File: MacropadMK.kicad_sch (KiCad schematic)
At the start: 43 parts, among them J1 BME280, SHT40 Module, J10 SCD40 Module, J11 Conn_01x03, J12 Conn_01x03, J13 SCD40 Module, J14 BME280, SHT40 Module, J15 mmWave Connector, J16 mmWave Connector, J17 mmWave Connector, J2 SCD40 Module, J3 Conn_01x02, J4 Qwiic_Vertical, J5 Conn_01x02, J6 Conn_01x02, J7 Conn_01x03, J8 Conn_01x03, J9 VL53L0X Module, Q1 PT19-21C, SW1 SW_Push, U5 TLP175A

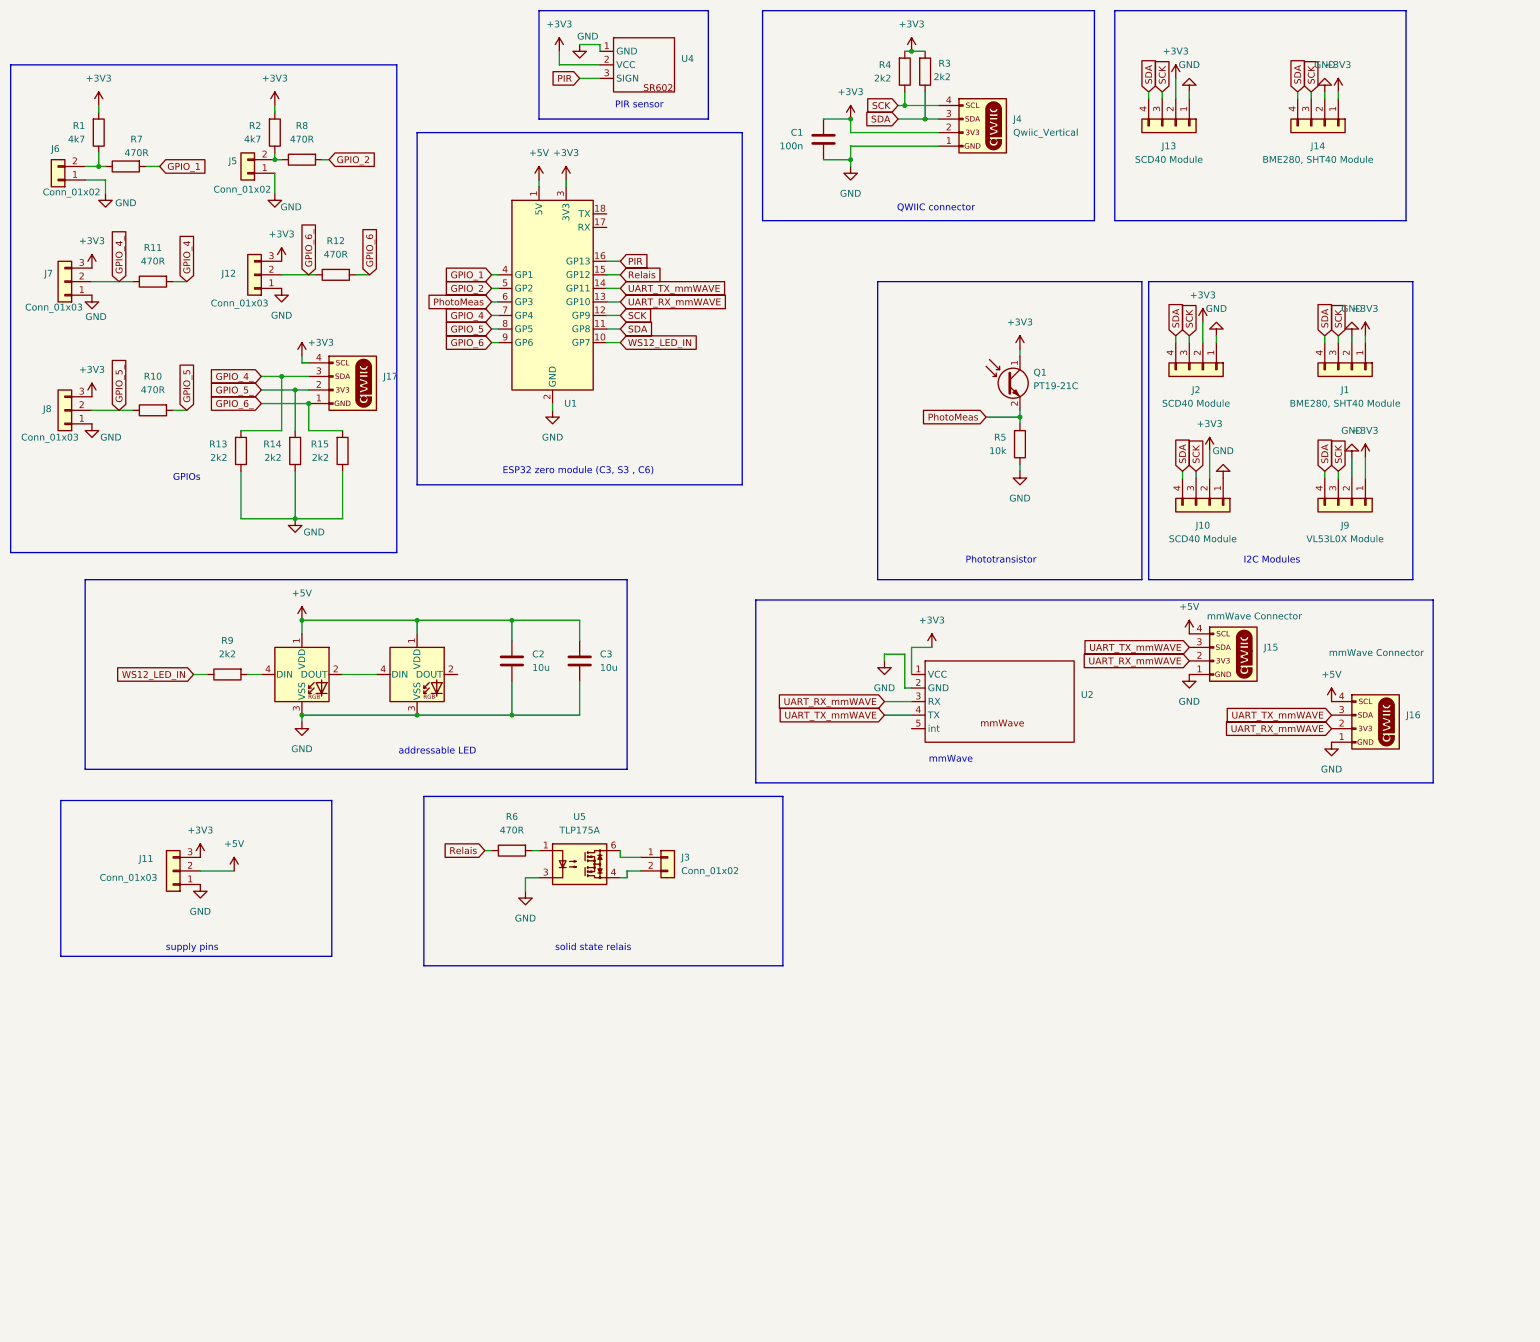
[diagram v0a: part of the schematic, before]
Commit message: added librarys
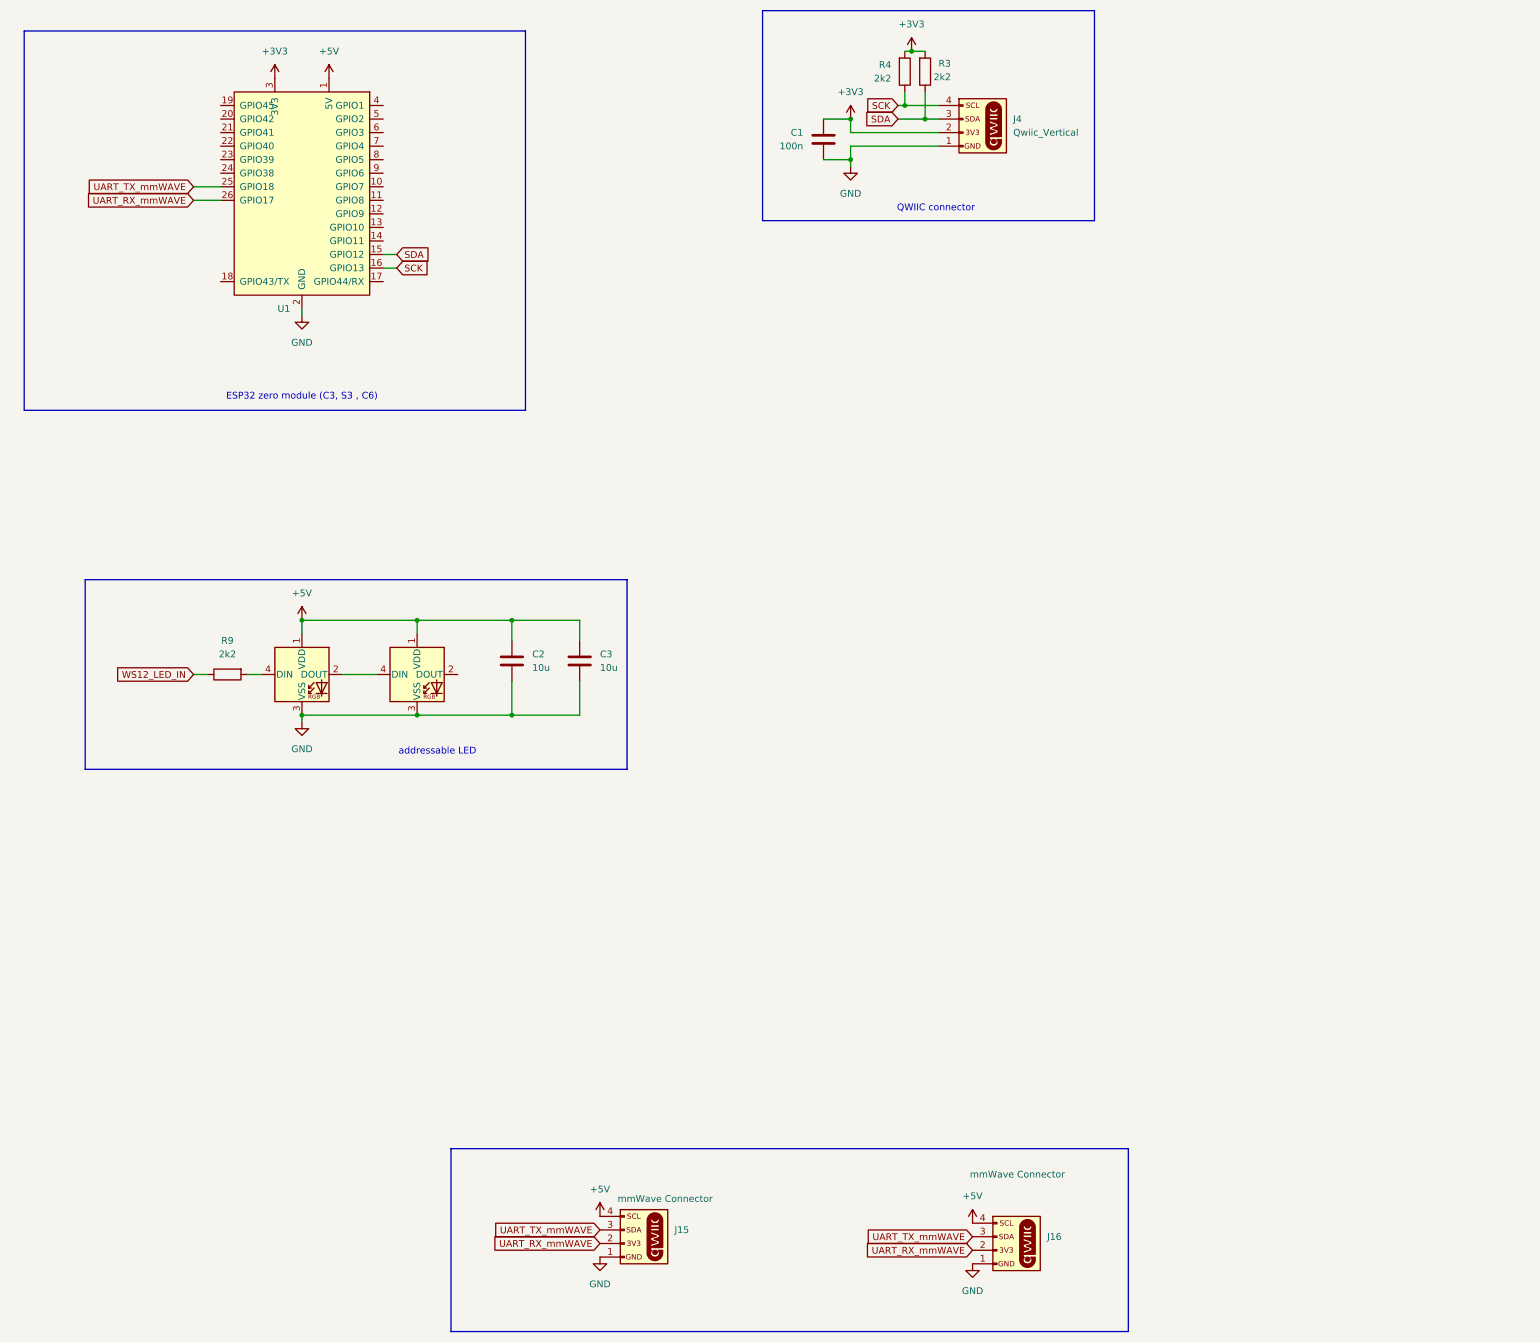
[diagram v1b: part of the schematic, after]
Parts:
- removed J1, J14: BME280, SHT40 Module, PCM_SparkFun-Connector:1x04_P2.54mm, symbol PCM_SparkFun-Connector:Conn_01x04_P2.54mm
- removed J10, J13, J2: SCD40 Module, PCM_SparkFun-Connector:1x04_P2.54mm, symbol PCM_SparkFun-Connector:Conn_01x04_P2.54mm
- removed J11, J12, J7, J8: Conn_01x03, PCM_SparkFun-Connector:1x03_P2.54mm, symbol PCM_SparkFun-Connector:Conn_01x03_P2.54mm
- removed J17: mmWave Connector, PCM_SparkFun-Connector:JST_1x04_P1.0mm_Vertical_SMD, symbol PCM_SparkFun-Connector:Qwiic_Vertical
- removed J3, J5, J6: Conn_01x02, PCM_SparkFun-Connector:1x02_P2.54mm, symbol PCM_SparkFun-Connector:Conn_01x02_P2.54mm
- removed J9: VL53L0X Module, PCM_SparkFun-Connector:1x04_P2.54mm, symbol PCM_SparkFun-Connector:Conn_01x04_P2.54mm
- removed Q1: PT19-21C, LED_SMD:LED_0603_1608Metric, symbol Device:Q_Photo_NPN
- removed R1, R2: 4k7, Resistor_SMD:R_0805_2012Metric, symbol Device:R
- removed R10, R11, R12, R6, R7, R8: 470R, Resistor_SMD:R_0805_2012Metric, symbol Device:R
- removed R13, R14, R15: 2k2, Resistor_SMD:R_0805_2012Metric, symbol Device:R
- removed R5: 10k, Resistor_SMD:R_0805_2012Metric, symbol Device:R
- removed U2: (no value), MacropadMK_Sensor_Footprints:HLK-LD2410B-mmWave-Sensor, symbol MacropadMK_Sensor_Symbols:HLK-LD2410B-mmWave-Sensor
- removed U4: (no value), MacropadMK_Sensor_Footprints:SR602-PIR-Motion-Sensor, symbol MacropadMK_Sensor_Symbols:SR602-PIR-Motion-Sensor
- removed U5: TLP175A, Package_SO:Toshiba_SOIC-4-6_4.4x3.6mm_P1.27mm, symbol Relay_SolidState:TLP175A
- U1: footprint MacropadMK_Custom_Footprints:ESP32-S3-Zero -> ProjectFootprints:ESP32-S3-Zero_Hybrid_BottomLabels
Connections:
- net PIR is gone; now on net SCK: U1.16 (GPIO13)
- net Relais is gone; now on net SDA: U1.15 (GPIO12)
- net SCK: no longer U1.12 (GP9)
- net SDA: no longer U1.11 (GP8)
- net UART_RX_mmWAVE: now also U1.26 (GPIO17); no longer U1.13 (GP10)
- net UART_TX_mmWAVE: now also U1.25 (GPIO18); no longer U1.14 (GP11)
- net WS12_LED_IN: no longer U1.10 (GP7)
- net GPIO_1: no longer names the net of U1.4 (GPIO1)
- net GPIO_2: no longer names the net of U1.5 (GPIO2)
- net GPIO_4: no longer names the net of U1.7 (GPIO4)
- net GPIO_5: no longer names the net of U1.8 (GPIO5)
- net GPIO_6: no longer names the net of U1.9 (GPIO6)
- net PhotoMeas: no longer names the net of U1.6 (GPIO3)
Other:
- note removed: "GPIOs"
- note removed: "I2C Modules"
- note removed: "PIR sensor"
- note removed: "Phototransistor"
- note removed: "mmWave"
- note removed: "solid state relais"
- note removed: "supply pins"
- moved on the sheet: J15, J16

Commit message: add librarys
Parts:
- added D3: 1N4148W, Diode_SMD:D_SOD-123, symbol Diode:1N4148W
- added SW2, SW3, SW4: SW_Push, Button_Switch_Keyboard:SW_Cherry_MX_1.00u_PCB, symbol Switch:SW_Push
- U1: footprint ProjectFootprints:ESP32-S3-Zero_Hybrid_BottomLabels -> MacropadMK_Custom_Footprints:ESP32-S3-Zero
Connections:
- net at SW1.2: now also D3.1 (K)
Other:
- moved on the sheet: C1, C2, C3, J4, R3, R4, R9, SW1
